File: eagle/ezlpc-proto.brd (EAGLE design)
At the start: 30.5 x 25.4 mm, 62 parts, among them J1 MICRO USB, Q1 12Mhz, T1 MMBT3906, U1 PRTR5V0U2X, U2 MIC5225-3.3v, U3 LPC11U35FHN33/501

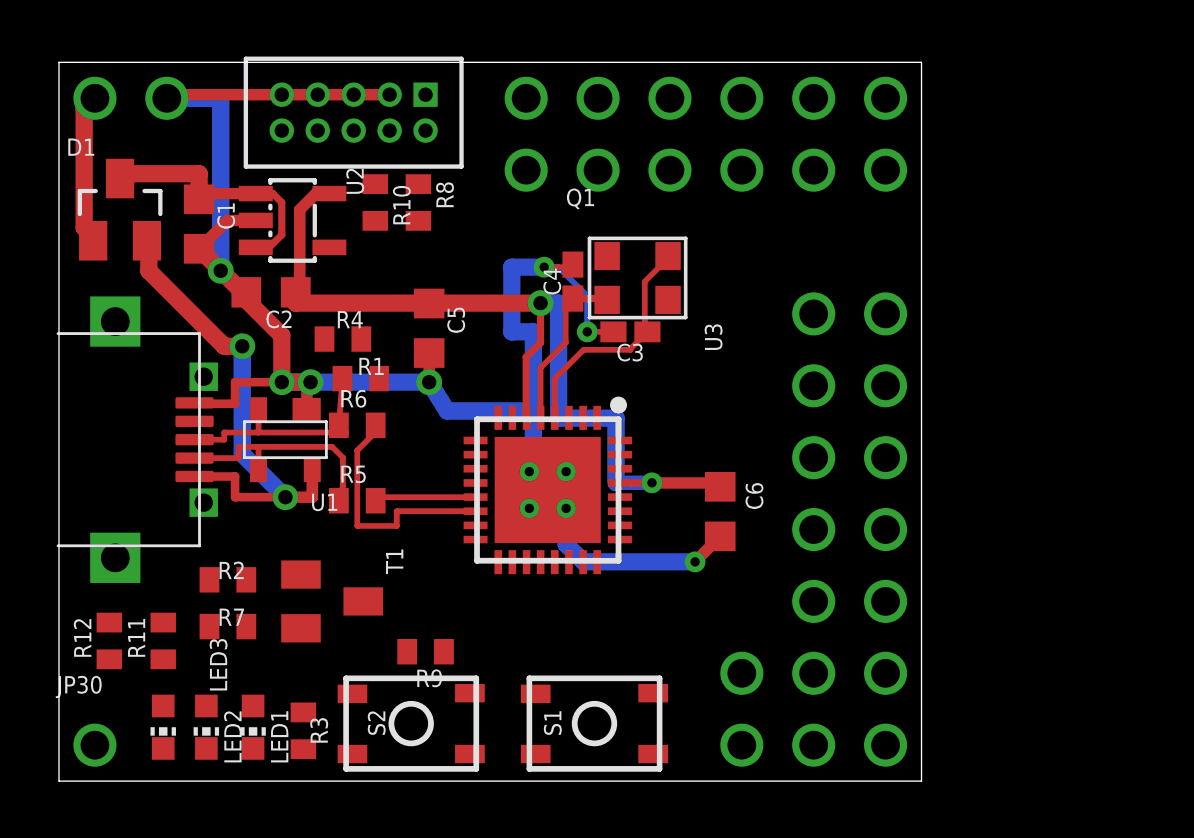
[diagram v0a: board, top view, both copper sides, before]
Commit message: Ready for final auto routing.
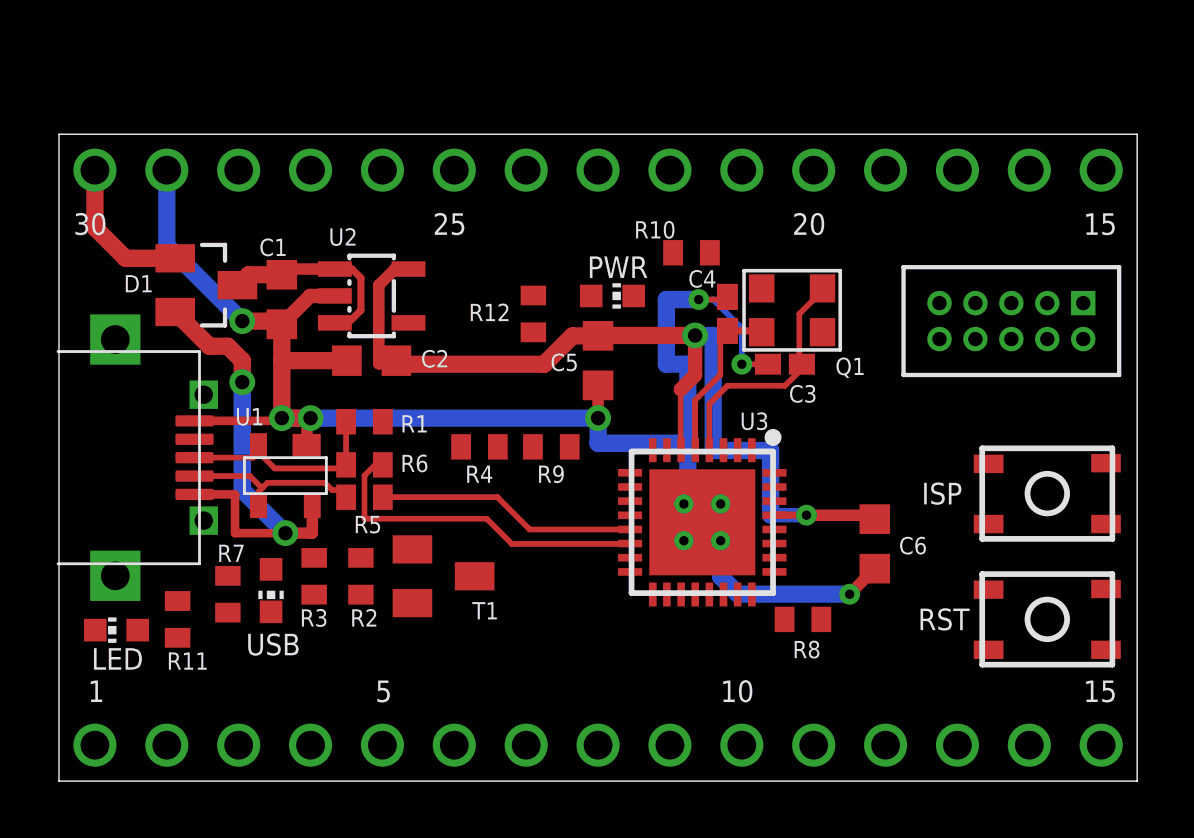
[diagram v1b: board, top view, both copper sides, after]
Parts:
- removed JP32: (no value), ezlpc-proto:1X01
- moved JP1 24.4 mm to (36.2, 16.9)
- moved S2 23.9 mm to (34.9, 10.2)
- moved JP23 22.9 mm to (3.81, 1.27)
- moved JP9 22.9 mm to (1.27, 1.27)
- moved LED3 22.0 mm to (19.6, 17.1), turned to 270 degrees
- moved JP30 20.5 mm to (3.81, 21.6)
- moved JP8 20.3 mm to (8.89, 1.27)
- moved R8 20.0 mm to (26.3, 5.71), turned to 180 degrees
- moved R12 18.9 mm to (16.8, 16.5), turned to 270 degrees
- moved JP10 18.0 mm to (6.35, 1.27)
- moved JP19 17.0 mm to (36.8, 1.27)
- moved S1 16.4 mm to (34.9, 5.71)
- moved JP11 15.5 mm to (11.4, 1.27)
- moved JP24 15.5 mm to (14.0, 1.27)
- moved JP26 14.8 mm to (34.3, 1.27)
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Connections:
- net GND: no longer JP32.1
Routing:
- net USB_DM: track 3.66 -> 9.22 mm
- net USB_DP: track 8.80 -> 12.5 mm
- net GND: track 68.1 -> 64.8 mm
- net +3V3: track 31.7 -> 34.0 mm
- net N$10: track 9.27 -> 7.27 mm
- net N$9: track 8.16 -> 6.50 mm
- net USB-5V: track 17.3 -> 16.3 mm
- net N$8: track 8.45 -> 7.62 mm
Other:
- board size 30.5 x 25.4 mm -> 38.1 x 22.9 mm
- board text added: "1"
- board text added: "10"
- board text added: "15"
- board text added: "20"
- board text added: "25"
- board text added: "30"
- board text added: "5"
- board text added: "ISP"
- board text added: "LED"
- board text added: "PWR"
- board text added: "RST"
- board text added: "USB"
